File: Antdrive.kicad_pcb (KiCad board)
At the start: 2 copper layers, 29 x 32 mm, 26 parts, among them J1 Conn_01x06, J2 Conn_01x03, M1 Conn_01x02, M2 Conn_01x02, Q1 MMBT3904, U2 STM32F030F4Px, U3 DRV8848, U5 HT75xx-1-SOT89

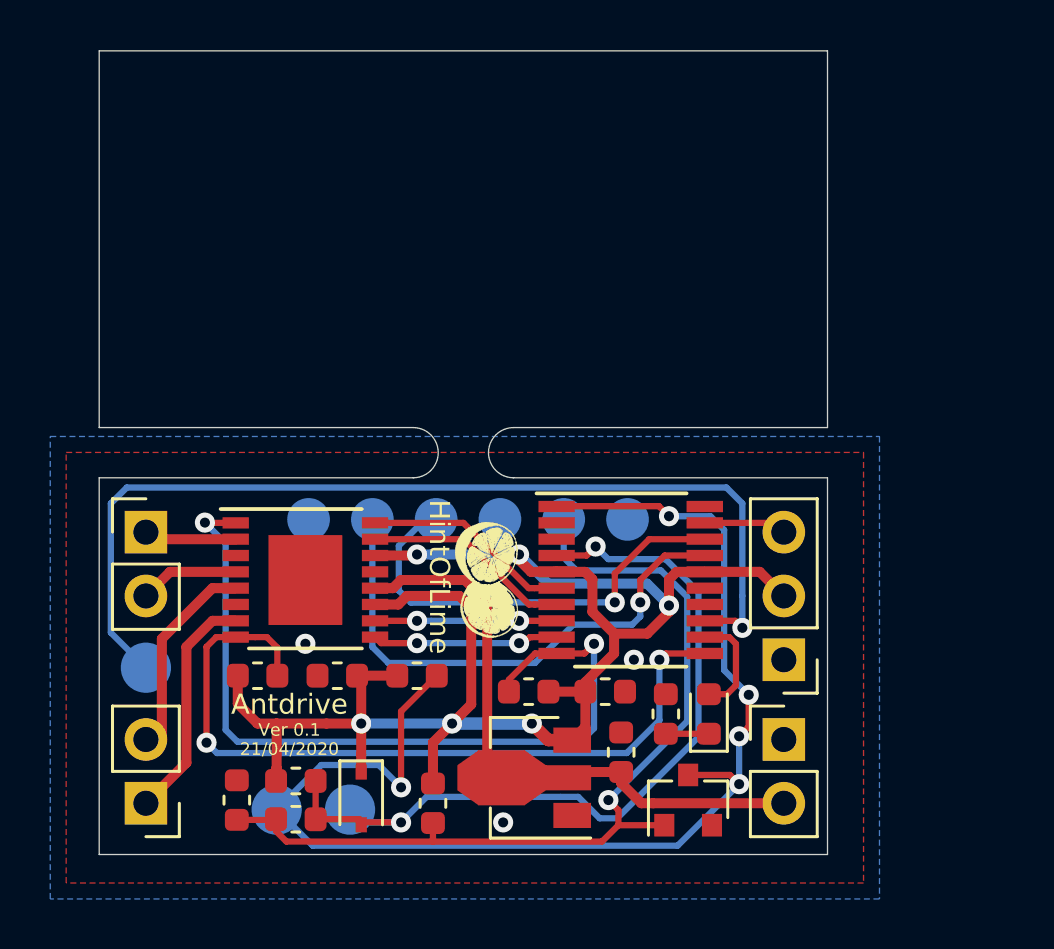
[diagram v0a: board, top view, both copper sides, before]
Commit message: PCB updated
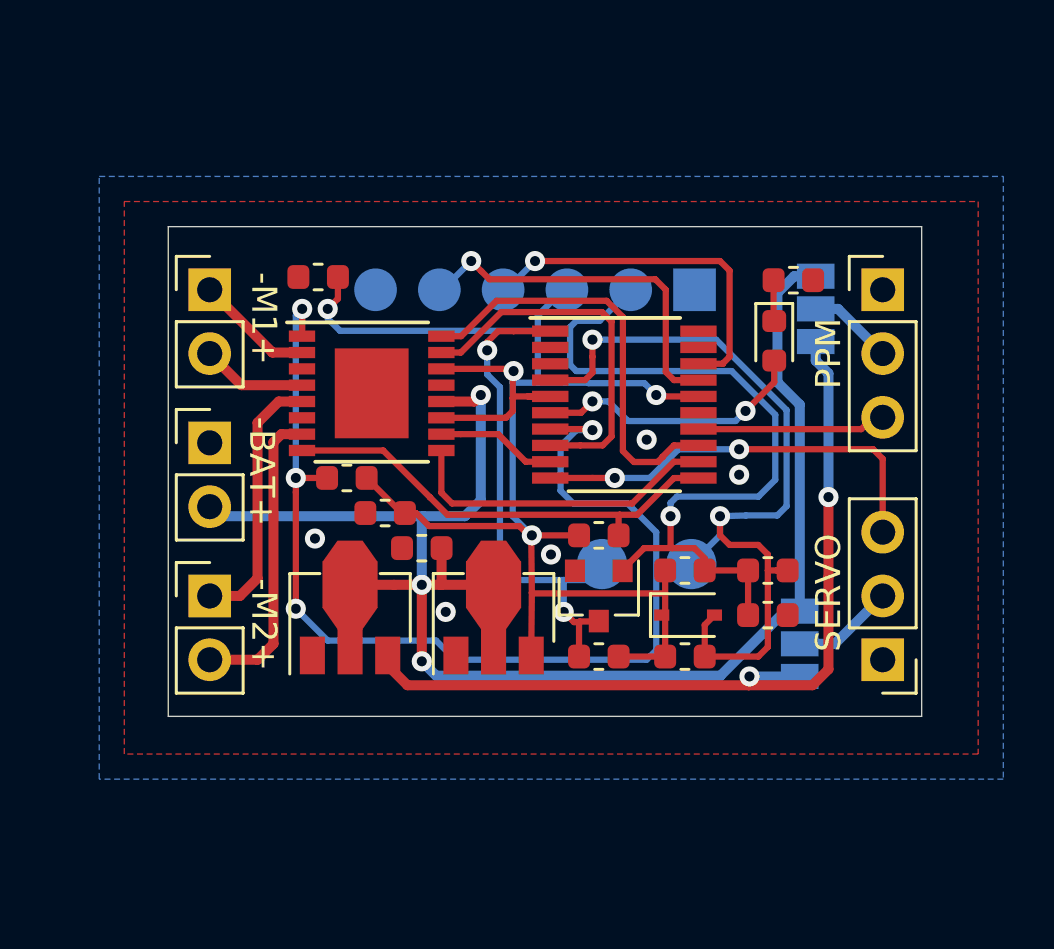
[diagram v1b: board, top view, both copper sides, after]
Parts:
- removed G***: LOGO, Symbol:lime_5mm
- removed TP3: Conn_01x01, TestPoint:TestPoint_Pad_D2.0mm
- added J3: Conn_01x03, Connector_PinHeader_2.54mm:PinHeader_1x03_P2.54mm_Vertical, F.Cu at (179.2, 55.2)
- added JP1: SolderJumper_3_Open, Jumper:SolderJumper-3_P1.3mm_Open_Pad1.0x1.5mm_NumberLabels, B.Cu at (176.5, 41.3)
- added JP2: SolderJumper_3_Open, Jumper:SolderJumper-3_P1.3mm_Open_Pad1.0x1.5mm_NumberLabels, B.Cu at (175.9, 54.6)
- added LOGO1: TestPoint, Symbol:lime_5mm, B.Cu at (161.2, 48.8)
- added U1: HT75xx-1-SOT89, Package_TO_SOT_SMD:SOT-89-3, F.Cu at (158.0, 53.6)
- moved BAT1 25.7 mm to (152.4, 46.6)
- moved R6 22.4 mm to (174.6, 53.5), turned to 0 degrees
- moved C4 21.2 mm to (174.6, 51.7)
- moved R4 18.0 mm to (175.6, 40.1), turned to 180 degrees
- moved TP2 16.7 mm to (171.6, 51.4)
- moved R7 16.3 mm to (171.3, 55.1)
- moved TP1 16.2 mm to (168.0, 51.4)
- moved C3 15.9 mm to (156.7, 40.0)
- moved J2 15.2 mm to (179.2, 40.5), turned to 0 degrees
- moved D1 15.1 mm to (174.9, 42.5), turned to 270 degrees
- moved D2 14.9 mm to (171.4, 53.5), turned to 0 degrees
- moved R3 14.7 mm to (167.9, 50.3)
- moved R1 13.7 mm to (171.3, 51.7), turned to 180 degrees
- moved C1 11.4 mm to (160.8, 50.8), turned to 180 degrees
- moved C2 11.3 mm to (159.4, 49.4), turned to 180 degrees
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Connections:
- J2 pad 2: +3V3 -> Net-(J2-Pad2)
- U2 pad 10: !SLEEP -> SERVO
- U2 pad 12: LED -> BIN1
- U2 pad 13: SERVO -> AIN1
- U2 pad 14: Net-(U2-Pad14) -> PPM
- U2 pad 19: PPM -> Net-(U2-Pad19)
- U2 pad 6: AIN1 -> LED
- U2 pad 7: AIN2 -> !SLEEP
- U2 pad 8: BIN2 -> AIN2
- U2 pad 9: BIN1 -> BIN2
- U3 pad 5: Net-(M2-Pad2) -> Net-(M2-Pad1)
- U3 pad 7: Net-(M2-Pad1) -> Net-(M2-Pad2)
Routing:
- net +BATT: track 24.4 -> 69.0 mm, vias 0 -> 3
- net +5V: track 0.00 -> 34.2 mm, vias 0 -> 2
- net BOOT: track 51.1 -> 20.6 mm, vias 5 -> 2
- net SERVO: track 39.4 -> 16.4 mm, vias 1 -> 2
- net !FAULT: track 31.2 -> 18.3 mm, vias 2 -> 0
- net !SLEEP: track 32.7 -> 43.9 mm, vias 2 -> 4
- net AIN1: track 8.31 -> 16.9 mm
- net LED: track 4.23 -> 10.9 mm, vias 0 -> 2
- net +3V3: track 71.3 -> 64.6 mm, vias 6 -> 4
- net RX: track 21.2 -> 14.7 mm
- net AIN2: track 8.31 -> 14.8 mm
- net CTS: track 36.7 -> 30.5 mm
- net BIN1: track 7.66 -> 12.8 mm, vias 2 -> 0
- net PPM: track 3.30 -> 7.53 mm
- net Net-(J3-Pad2): track 0.00 -> 4.09 mm
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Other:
- board size 29 x 32 mm -> 30 x 19.5 mm
- board text added: "-BAT+"
- board text added: "-M1+"
- board text added: "-M2+"
- board text added: "BAT/5V"
- board text added: "Ver 0.2"
- board text removed: "BAT+"
- board text removed: "BAT-"
- board text removed: "M1"
- board text removed: "M2"
- board text removed: "Ver 0.1"
